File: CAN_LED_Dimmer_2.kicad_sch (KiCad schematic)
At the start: 25 parts, among them J6 CON_4P_1190299, Q7 Q_IPD90P04P4L04ATMA2, Q8 Q_IPD90P04P4L04ATMA2, U4 U_LM5166XDRCR

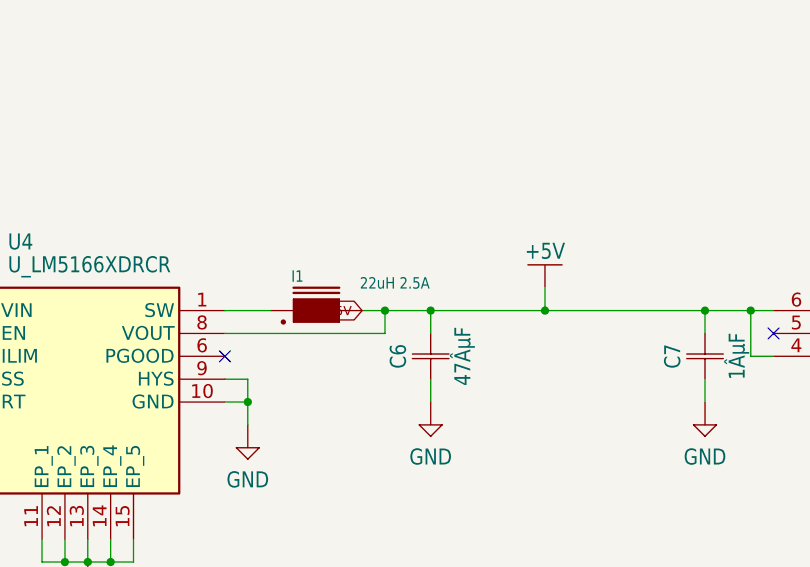
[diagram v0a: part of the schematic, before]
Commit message: Further layout
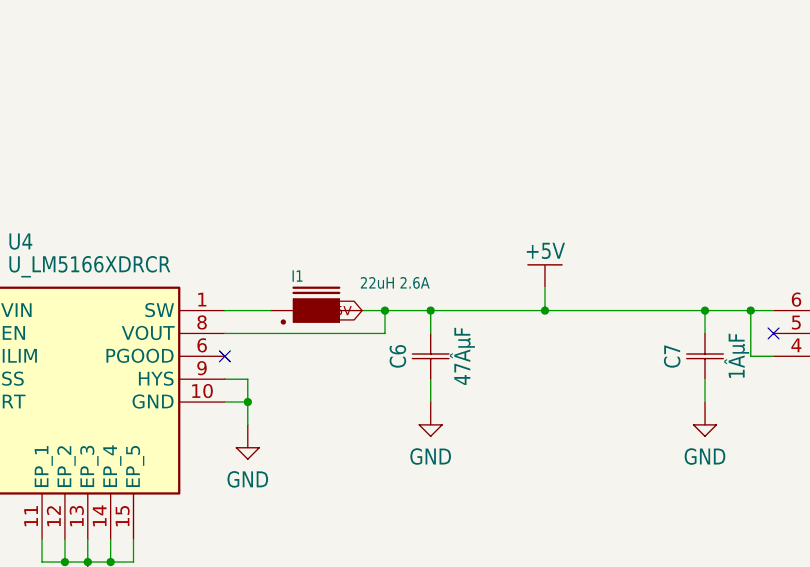
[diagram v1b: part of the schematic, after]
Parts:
- I1: value 22uH 2.5A -> 22uH 2.6A; footprint CAN_LED_Dimmer-layout:INDM7166X300N_ASPI-0630LR_I1 -> CAN_LED_Dimmer-layout:SMMS0630-220M_I1; symbol CAN LED Dimmer-eagle-import:IND_ASPI-0630LR-220M-T15 -> CAN LED Dimmer-eagle-import:IND_SMMS0630-220M; MANUFACTURER Abracon -> SXN (Shun Xiang Nuo); MPN ASPI-0630LR-220M-T15 -> SMMS0630-220M
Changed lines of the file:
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@@
 	)
 	(symbol
-		(lib_id "CAN LED Dimmer-eagle-import:IND_ASPI-0630LR-220M-T15")
+		(lib_id "CAN LED Dimmer-eagle-import:IND_SMMS0630-220M")
 		(at 149.86 185.42 0)
 		(unit 1)
@@
 			)
 		)
-		(property "Value" "22uH 2.5A"
+		(property "Value" "22uH 2.6A"
 			(at 154.686 183.134 0)
 			(show_name no)
@@
 			)
 		)
-		(property "Footprint" "CAN_LED_Dimmer-layout:INDM7166X300N_ASPI-0630LR_I1"
+		(property "Footprint" "CAN_LED_Dimmer-layout:SMMS0630-220M_I1"
 			(at 149.86 185.42 0)
 			(hide yes)
@@
 			)
 		)
-		(property "Datasheet" ""
+		(property "Datasheet" "https://www.lcsc.com/datasheet/C128694.pdf"
 			(at 149.86 185.42 0)
 			(hide yes)
@@
 			)
 		)
-		(property "Description" ""
+		(property "Description" "Shielded 22uH, DCR 135mOhm max, Isat 3.5A typ; LCSC C128694"
 			(at 149.86 185.42 0)
 			(hide yes)
@@
 			)
 		)
-		(property "MANUFACTURER" "Abracon"
+		(property "MANUFACTURER" "SXN (Shun Xiang Nuo)"
 			(at 149.86 192.786 0)
 			(hide yes)
@@
 			)
 		)
-		(property "MPN" "ASPI-0630LR-220M-T15"
+		(property "MPN" "SMMS0630-220M"
 			(at 149.86 194.31 0)
 			(hide yes)

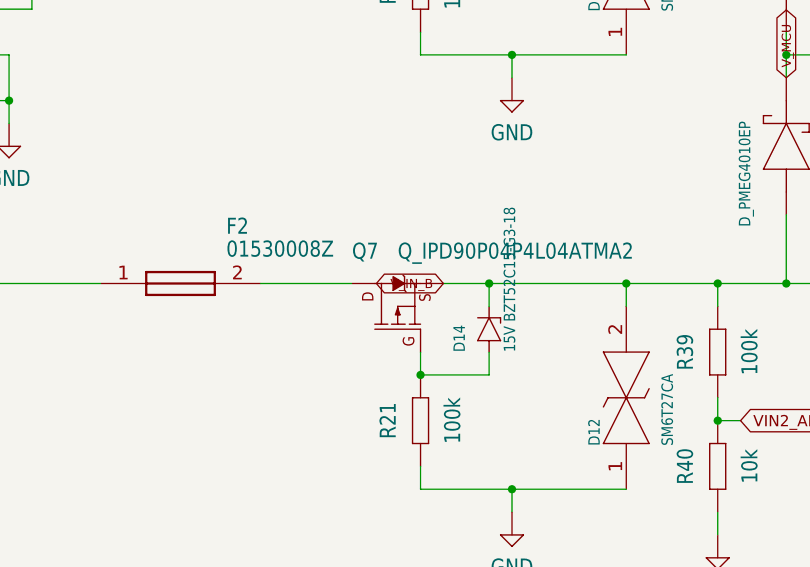
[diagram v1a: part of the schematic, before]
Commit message: modified rules
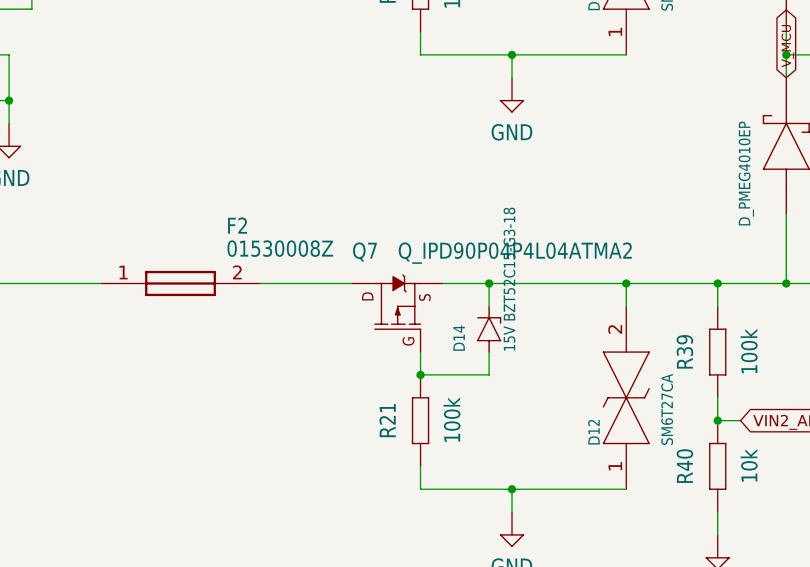
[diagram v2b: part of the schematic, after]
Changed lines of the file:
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@@
 	(generator_version "10.0")
 	(paper "User" 425.45 298.6024)
+	(text "F1 / F2: MINI-Sicherungshalter; Bestueckung mit je 10-A-Sicherung."
+		(exclude_from_sim no)
+		(at 30 265 0)
+		(effects
+			(font
+				(size 1.27 1.27)
+			)
+			(justify left)
+		)
+	)
 	(junction
 		(at 127 213.36)
@@
 		(color 0 0 0 0)
 	)
+	(no_connect
+		(at 139.7 190.5)
+	)
+	(no_connect
+		(at 109.22 193.04)
+	)
+	(no_connect
+		(at 200.66 187.96)
+	)
+	(no_connect
+		(at 236.22 187.96)
+	)
 	(wire
 		(pts
@@
 		)
 	)
-	(global_label "V_IN_B"
-		(shape bidirectional)
-		(at 170.18 101.6 180)
-		(fields_autoplaced yes)
-		(effects
-			(font
-				(size 1.016 1.016)
-			)
-			(justify right)
-		)
-		(property "Intersheetrefs" "${INTERSHEET_REFS}"
-			(at 161.9198 101.6 0)
-			(hide yes)
-			(show_name no)
-			(do_not_autoplace no)
-			(effects
-				(font
-					(size 1.27 1.27)
-				)
-				(justify right)
-			)
-		)
-	)
 	(symbol
 		(lib_id "CAN LED Dimmer-eagle-import:GND")
@@
 		)
 	)
-(text "F1 / F2: MINI-Sicherungshalter; Bestueckung mit je 10-A-Sicherung."
- (at 30 265 0) (effects (font (size 1.27 1.27)) (justify left)))
-(no_connect (at 109.22 193.04))
-(no_connect (at 139.7 190.5))
-(no_connect (at 200.66 187.96))
-(no_connect (at 236.22 187.96))
 )

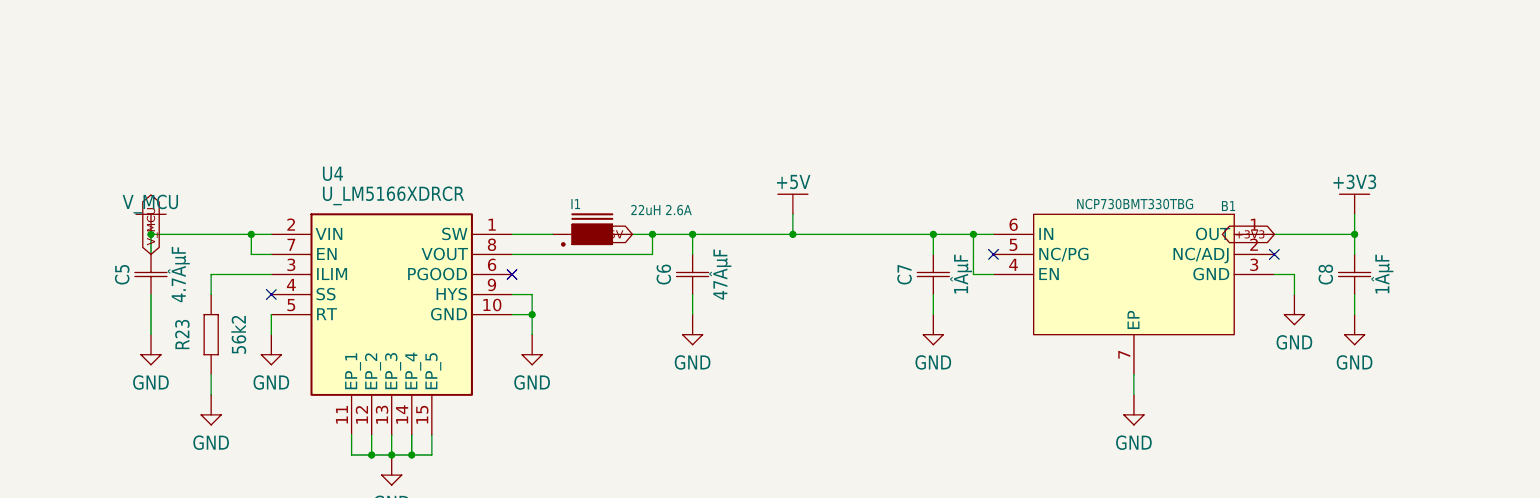
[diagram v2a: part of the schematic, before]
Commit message: further layouten
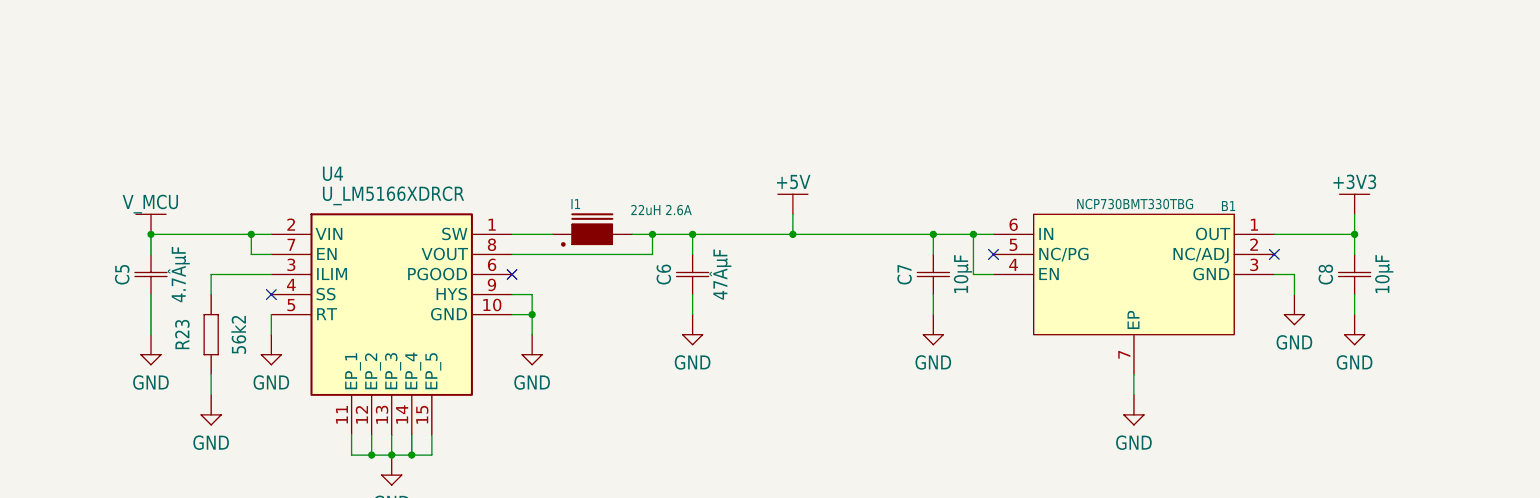
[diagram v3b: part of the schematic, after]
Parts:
- C7, C8: value 1ÂµF -> 10µF
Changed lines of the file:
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@@
 		)
 	)
-	(global_label "V_MCU"
-		(shape bidirectional)
-		(at 93.98 187.96 90)
-		(fields_autoplaced yes)
-		(effects
-			(font
-				(size 1.016 1.016)
-			)
-			(justify left)
-		)
-		(property "Intersheetrefs" "${INTERSHEET_REFS}"
-			(at 93.98 179.7966 90)
-			(hide yes)
-			(show_name no)
-			(do_not_autoplace no)
-			(effects
-				(font
-					(size 1.27 1.27)
-				)
-				(justify left)
-			)
-		)
-	)
-	(global_label "+3V3"
-		(shape bidirectional)
-		(at 236.22 185.42 180)
-		(fields_autoplaced yes)
-		(effects
-			(font
-				(size 1.016 1.016)
-			)
-			(justify right)
-		)
-		(property "Intersheetrefs" "${INTERSHEET_REFS}"
-			(at 228.8791 185.42 0)
-			(hide yes)
-			(show_name no)
-			(do_not_autoplace no)
-			(effects
-				(font
-					(size 1.27 1.27)
-				)
-				(justify right)
-			)
-		)
-	)
 	(global_label "V_IN_A"
 		(shape bidirectional)
@@
 		)
 	)
-	(global_label "+5V"
-		(shape bidirectional)
-		(at 154.94 185.42 180)
-		(fields_autoplaced yes)
-		(effects
-			(font
-				(size 1.016 1.016)
-			)
-			(justify right)
-		)
-		(property "Intersheetrefs" "${INTERSHEET_REFS}"
-			(at 148.5667 185.42 0)
-			(hide yes)
-			(show_name no)
-			(do_not_autoplace no)
-			(effects
-				(font
-					(size 1.27 1.27)
-				)
-				(justify right)
-			)
-		)
-	)
 	(symbol
 		(lib_id "CAN LED Dimmer-eagle-import:GND")
@@
 			)
 		)
-		(property "Value" "1ÂµF"
+		(property "Value" "10µF"
 			(at 248.92 190.5 0)
 			(show_name no)
@@
 			)
 		)
-		(property "Value" "1ÂµF"
+		(property "Value" "10µF"
 			(at 195.58 190.5 0)
 			(show_name no)
